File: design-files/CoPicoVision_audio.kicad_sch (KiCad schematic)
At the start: 7 parts, among them J501 AudioJack3, Q501 KSD1616A, U501 SN76489AN

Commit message: Use a vertical footprint for R501.
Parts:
- R501: footprint Resistor_THT:R_Axial_DIN0204_L3.6mm_D1.6mm_P5.08mm_Horizontal -> Resistor_THT:R_Axial_DIN0207_L6.3mm_D2.5mm_P2.54mm_Vertical
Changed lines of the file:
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@@
       (effects (font (size 1.27 1.27)) (justify left))
     )
-    (property "Footprint" "Resistor_THT:R_Axial_DIN0204_L3.6mm_D1.6mm_P5.08mm_Horizontal" (at 116.332 95.885 0)
+    (property "Footprint" "Resistor_THT:R_Axial_DIN0207_L6.3mm_D2.5mm_P2.54mm_Vertical" (at 116.332 95.885 0)
       (effects (font (size 1.27 1.27)) hide)
     )

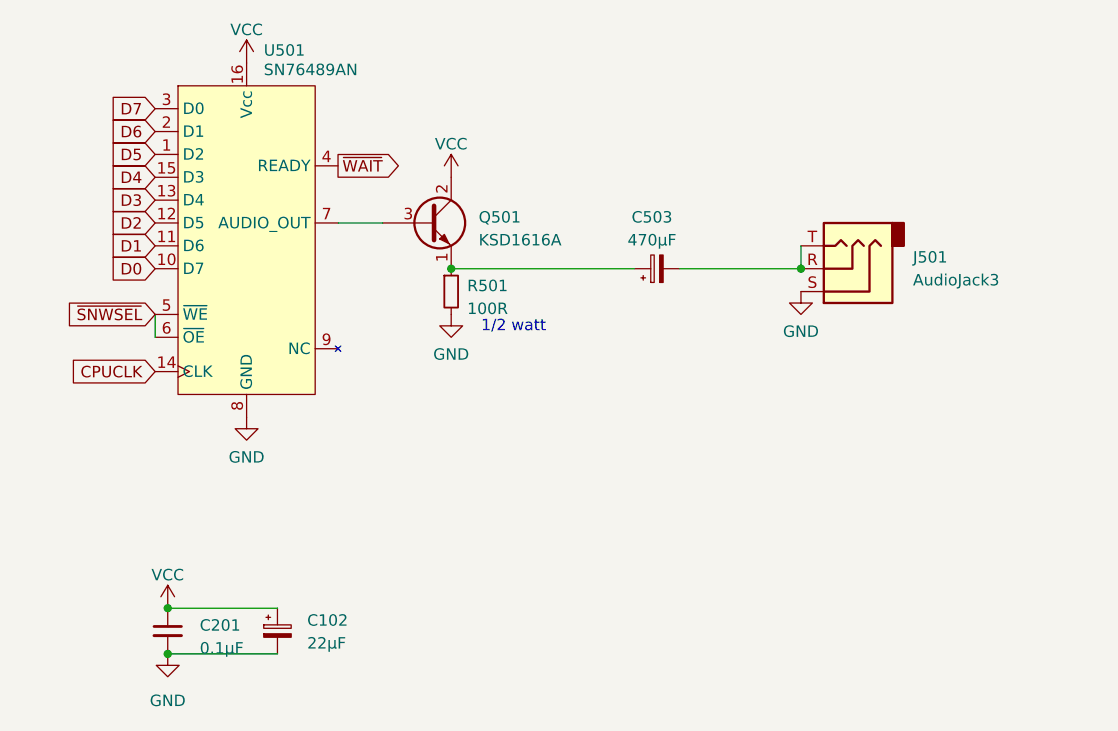
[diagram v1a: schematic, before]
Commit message: Add a 1.5K current limiting resistor between the SN76489AN audio output and the KSD1616A emitter-follower.
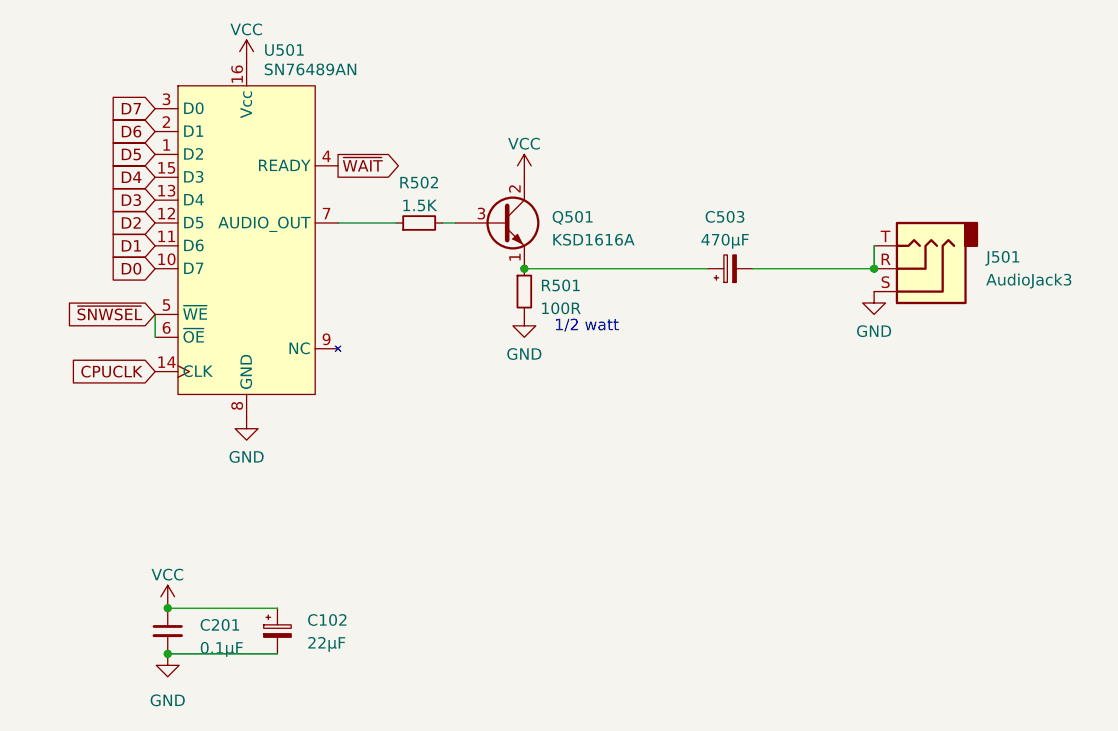
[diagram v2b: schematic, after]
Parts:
- added R502: 1.5K, Resistor_THT:R_Axial_DIN0207_L6.3mm_D2.5mm_P2.54mm_Vertical, symbol Device:R_Small
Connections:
- net at Q501.3 (B): now also R502.2; no longer U501.7 (AUDIO_OUT)
- new net: R502.1, U501.7 (AUDIO_OUT)
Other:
- moved on the sheet: C503, J501, Q501, R501
